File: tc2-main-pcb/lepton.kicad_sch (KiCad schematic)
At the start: 31 parts, among them U113 3N25000G33YC, U114 Flir_LEPTON, U118 TLV75530PDRV, U119 TLV75528PDRV, U120 TPS62A02DRLR

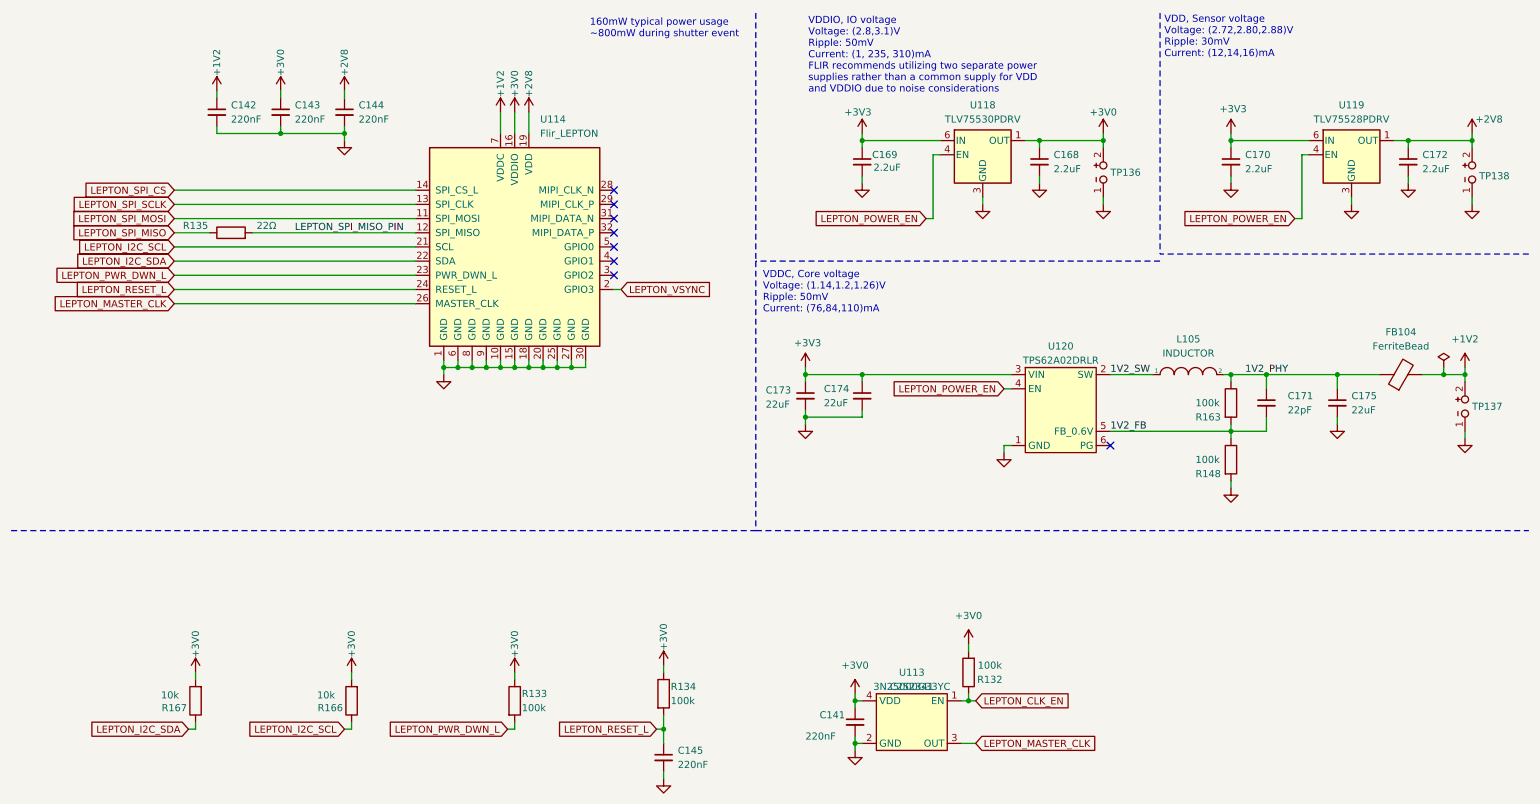
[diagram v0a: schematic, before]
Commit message: Update schematic
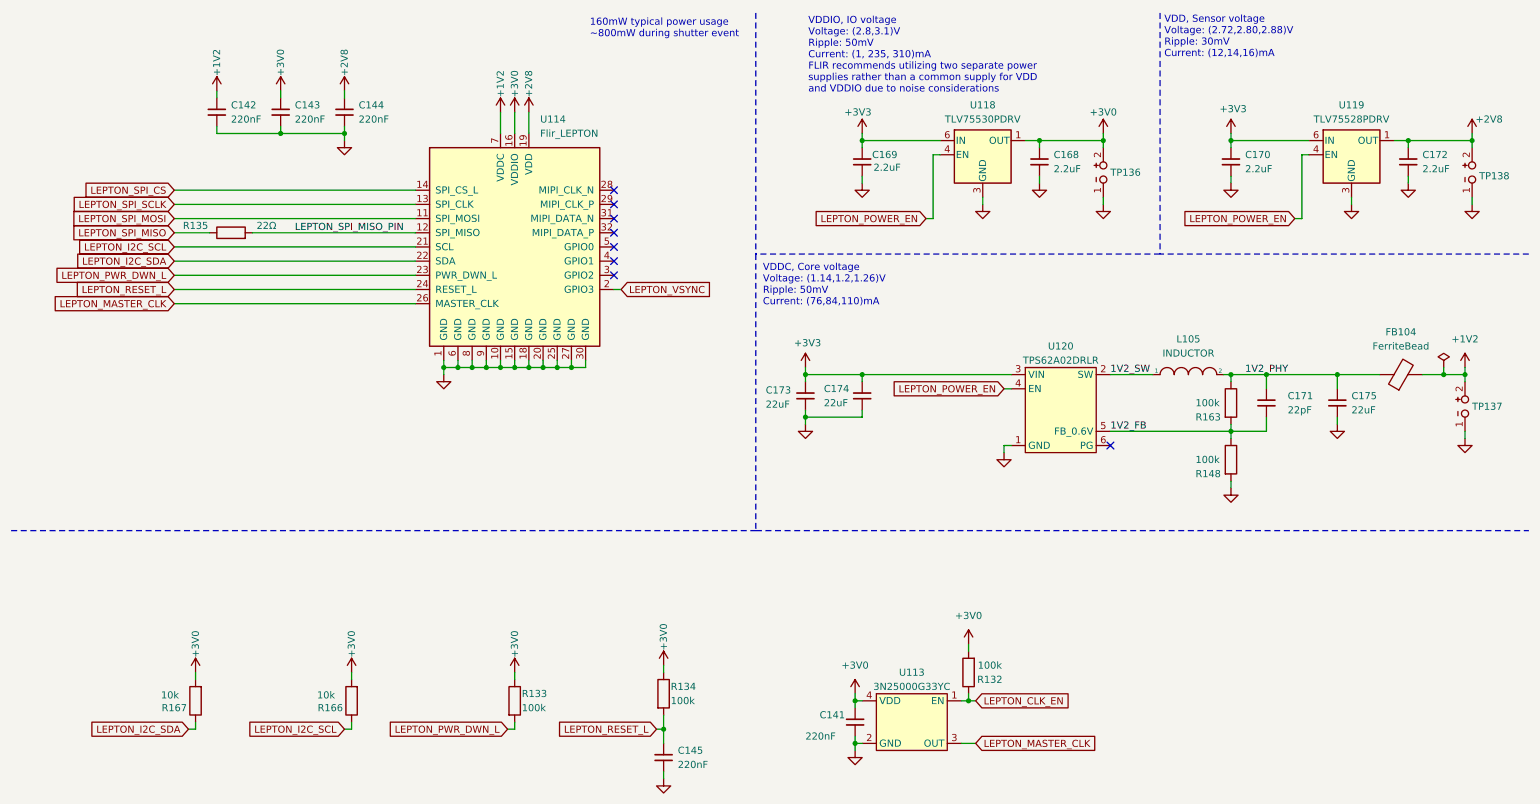
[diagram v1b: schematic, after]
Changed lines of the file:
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@@
 	(text "VDDC, Core voltage\nVoltage: (1.14,1.2,1.26)V\nRipple: 50mV\nCurrent: (76,84,110)mA"
 		(exclude_from_sim no)
-		(at 147.32 66.548 0)
+		(at 147.32 65.278 0)
 		(effects
 			(font
@@
 	(polyline
 		(pts
-			(xy 218.44 57.15) (xy 146.05 57.15)
+			(xy 218.44 55.88) (xy 146.05 55.88)
 		)
 		(stroke
@@
 	(polyline
 		(pts
-			(xy 146.05 12.7) (xy 146.05 57.15)
+			(xy 146.05 12.7) (xy 146.05 55.88)
 		)
 		(stroke
@@
 	(polyline
 		(pts
-			(xy 146.05 57.15) (xy 146.05 105.41)
+			(xy 146.05 55.88) (xy 146.05 105.41)
 		)
 		(stroke
@@
 		(property "LCSC Part" "C252341"
 			(at 173.99 133.35 0)
+			(hide yes)
 			(show_name no)
 			(do_not_autoplace no)
